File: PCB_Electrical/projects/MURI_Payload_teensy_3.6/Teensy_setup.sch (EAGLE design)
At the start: 53 parts, among them IC1 DS18B20, IC2 DS18B20, IC3 74ALS08N, IC4 DS18B20, IC5 DS18B20, U1 ADXL345

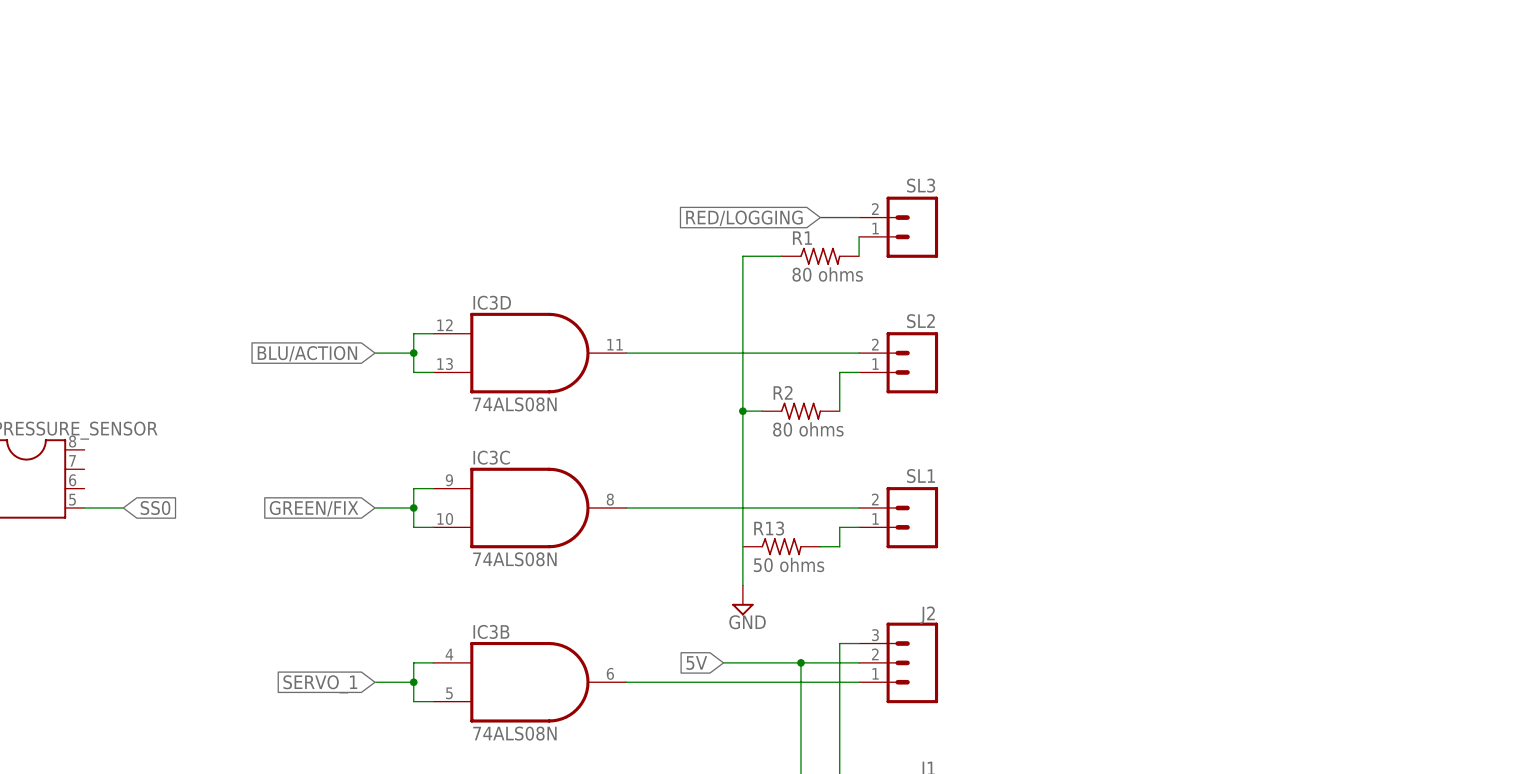
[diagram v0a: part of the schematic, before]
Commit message: Added changes, don't know what they were lol
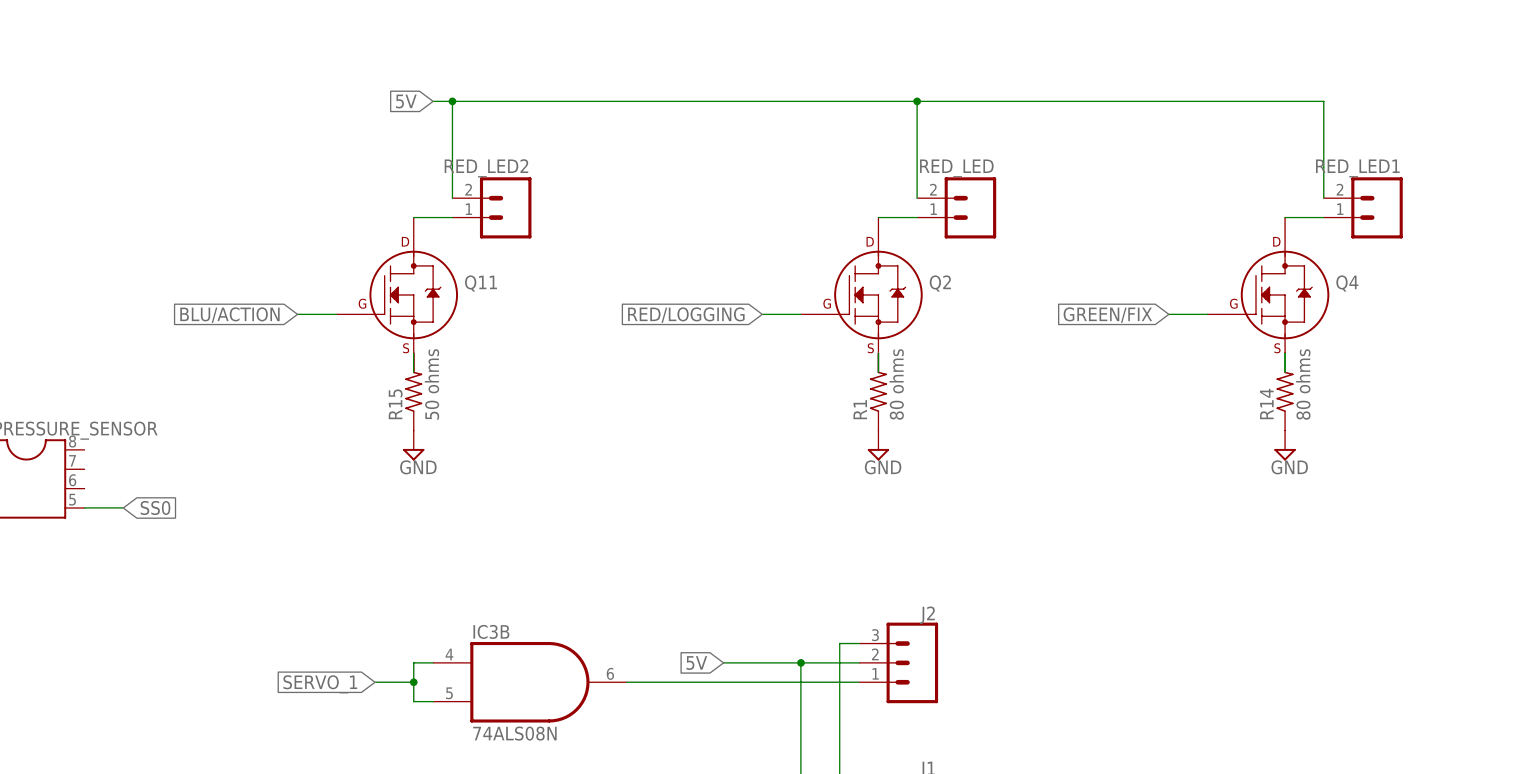
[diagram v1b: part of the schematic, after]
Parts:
- removed R13: 50 ohms, resistor:R-US_0207/7
- removed R2: 80 ohms, resistor:R-US_0207/7
- removed SL1, SL2, SL3: (no value), con-amp-quick:M02
- added Q11, Q2, Q4: (no value), transistors:2N7000_TO92
- added R14: 80 ohms, resistor:R-US_0207/7
- added R15: 50 ohms, resistor:R-US_0207/7
- added RED_LED, RED_LED1, RED_LED2: (no value), con-amp-quick:M02
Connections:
- removed net N$2: R2.2, SL2.1
- removed net N$3: R13.2, SL1.1
- removed net N$7: IC3C.O, SL1.2
- new net N$16: Q4.D, RED_LED1.1
- new net N$17: Q11.S, R15.2
- new net N$18: Q11.D, RED_LED2.1
- new net N$5: Q2.D, RED_LED.1
- net 5V: now also RED_LED.2, RED_LED1.2, RED_LED2.2
- net BLU/ACTION: now also Q11.G; no longer IC3D.I0, IC3D.I1
- net GND: now also R14.1, R15.1; no longer R2.1
- net GREEN/FIX: now also Q4.G; no longer IC3C.I0, IC3C.I1
- net N$4: now also Q2.S; no longer SL3.1
- net N$6: now also Q4.S, R14.2; no longer IC3D.O, SL2.2
- net RED/LOGGING: now also Q2.G; no longer SL3.2
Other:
- moved on the sheet: R1
